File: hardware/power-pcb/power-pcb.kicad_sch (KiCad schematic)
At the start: 28 parts, among them J1 MicroFit3.0_1x2, J2 XT60PW-M-AS, J3 XT30, J4 XT30, K1 CB1-P-12V, Q1 SI4946CDY-T1-GE3, Q2 IRF4905, U1 LTC4365TS8, U2 TMCS1100A2QDR

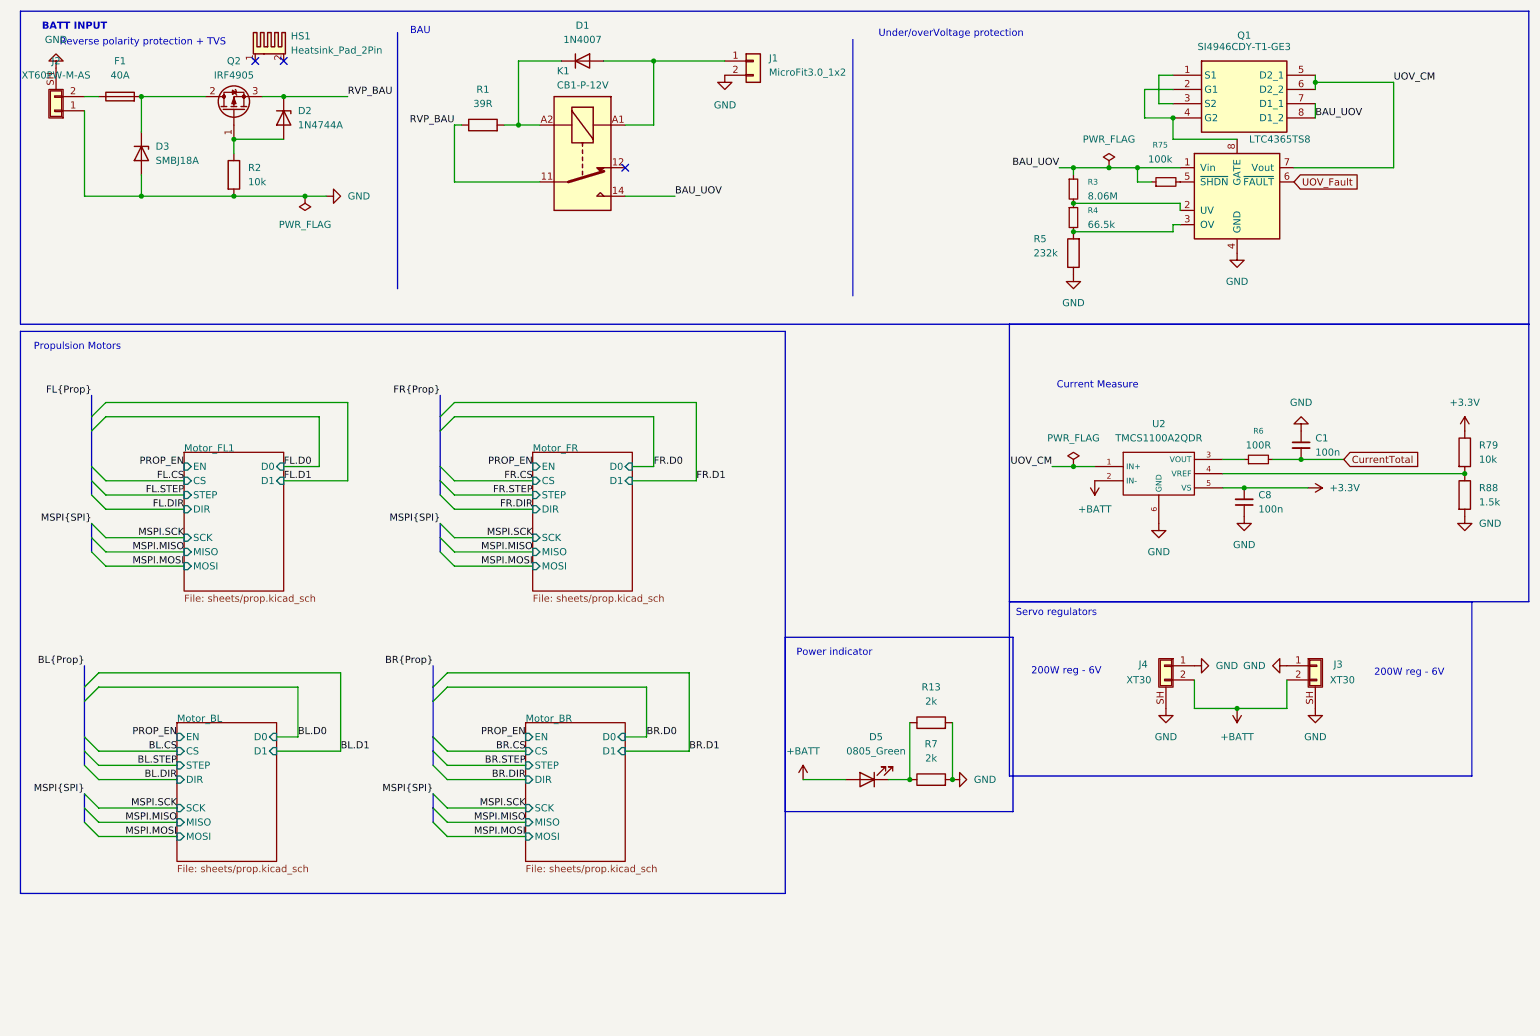
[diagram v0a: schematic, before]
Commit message: Added power pcb sch + design
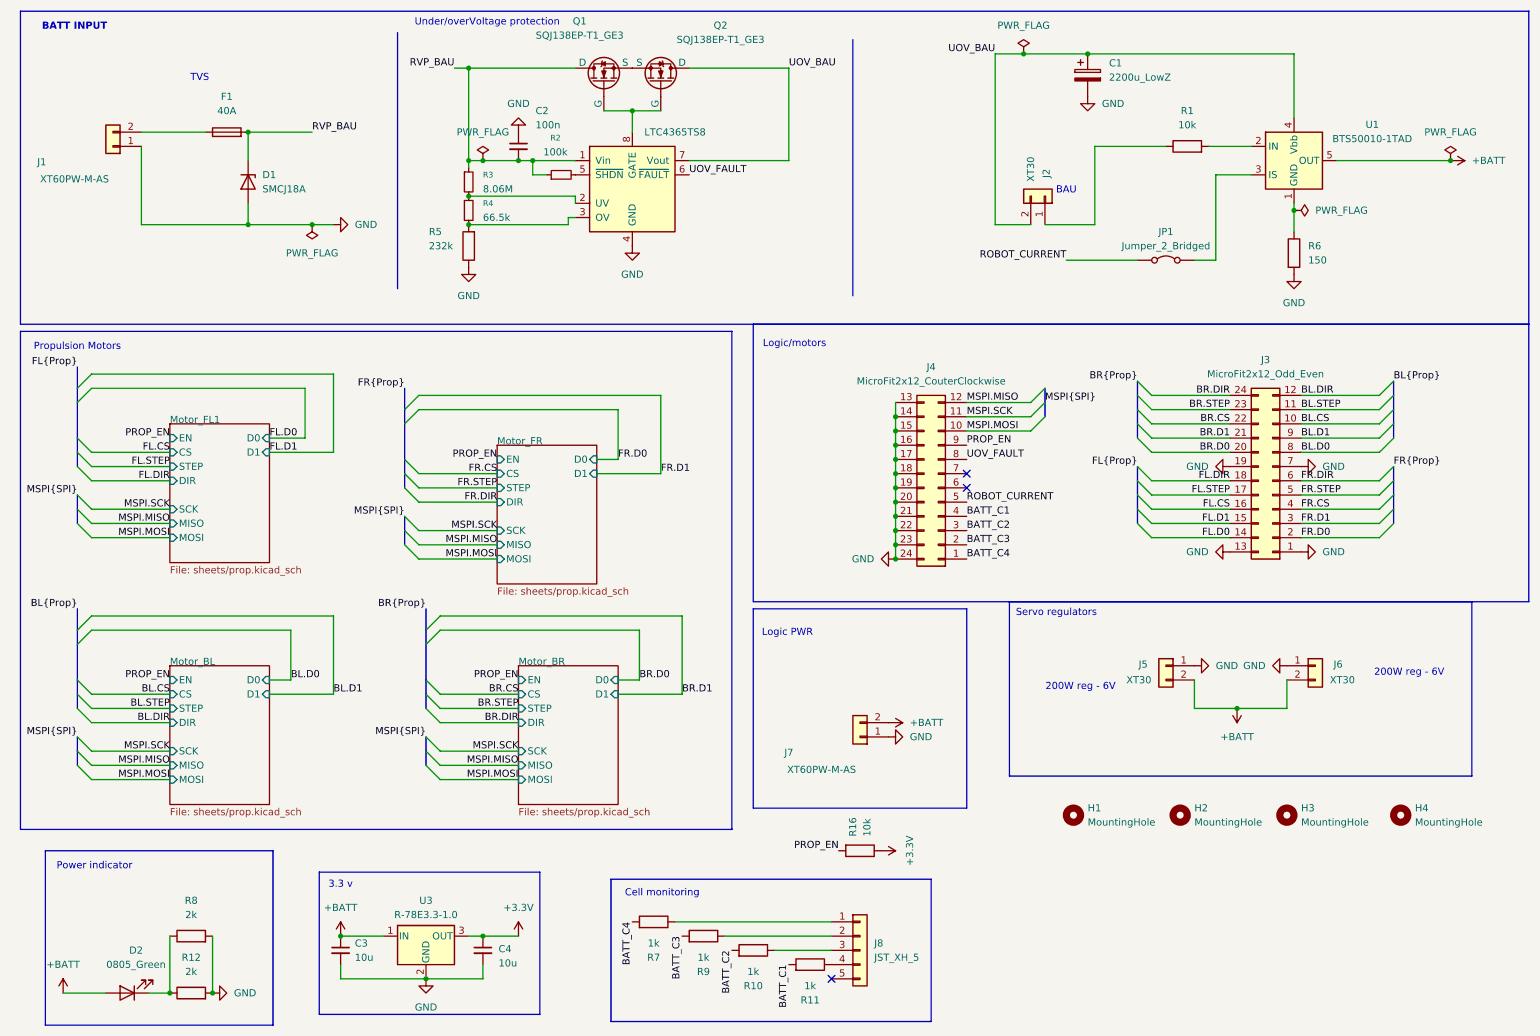
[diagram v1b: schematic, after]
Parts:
- removed C1, C8: 100n, Capacitor_SMD:C_0805_2012Metric_Pad1.18x1.45mm_HandSolder, symbol Device:C_Small
- removed D1: 1N4007, Diode_THT:D_DO-41_SOD81_P10.16mm_Horizontal, symbol Diode:1N4007
- removed D2: 1N4744A, Diode_THT:D_DO-41_SOD81_P10.16mm_Horizontal, symbol Diode:1N47xxA
- removed HS1: Heatsink_Pad_2Pin, Project:265118ABHE22, symbol Mechanical:Heatsink_Pad_2Pin
- removed J1: MicroFit3.0_1x2, Project:Molex_Micro-Fit_3.0_43650-0215_1x02_P3.00mm_Vertical, symbol Connector_Generic:Conn_01x02
- removed K1: CB1-P-12V, Project:CB1P12V, symbol Relay:Relay_SPDT
- removed Q1: SI4946CDY-T1-GE3, Package_SO:SO-8_3.9x4.9mm_P1.27mm, symbol Project:SISB46DN-T1-GE3
- removed Q2: IRF4905, Package_TO_SOT_THT:TO-220-3_Vertical, symbol Transistor_FET:IRF4905
- removed R2, R79: 10k, Resistor_SMD:R_0805_2012Metric_Pad1.20x1.40mm_HandSolder, symbol Device:R
- removed R6: 100R, Resistor_SMD:R_0805_2012Metric_Pad1.20x1.40mm_HandSolder, symbol Device:R_Small
- removed R88: 1.5k, Resistor_SMD:R_0805_2012Metric_Pad1.20x1.40mm_HandSolder, symbol Device:R
- removed U2: TMCS1100A2QDR, Project:TMCS1100A2QDR, symbol Project:TMCS1100A2QDR
- added C1: 2200u_LowZ, Capacitor_THT:CP_Radial_D16.0mm_P7.50mm, symbol Device:C_Polarized
- added C2: 100n, Capacitor_SMD:C_0805_2012Metric_Pad1.18x1.45mm_HandSolder, symbol Device:C_Small
- added C3, C4: 10u, Capacitor_SMD:C_0805_2012Metric_Pad1.18x1.45mm_HandSolder, symbol Device:C_Small
- added H1, H2, H3, H4: MountingHole, MountingHole:MountingHole_3.2mm_M3, symbol Mechanical:MountingHole
- added J2: XT30, Project:AMASS_XT30UPB-M_1x02_P5.0mm_Vertical, symbol Connector_Generic:Conn_01x02
- added J3: MicroFit2x12_Odd_Even, Project:Molex_Micro-Fit_3.0_43045-2412_2x12_P3.00mm_Vertical, symbol Connector_Generic:Conn_02x12_Top_Bottom
- added J4: MicroFit2x12_CouterClockwise, Project:Molex_Micro-Fit_3.0_43045-2412_2x12_P3.00mm_Vertical, symbol Connector_Generic:Conn_02x12_Counter_Clockwise
- added J7: XT60PW-M-AS, Connector_AMASS:AMASS_XT60-M_1x02_P7.20mm_Vertical, symbol Connector_Generic:Conn_01x02
- added J8: JST_XH_5, Project:JST_XH_B5B-XH-AM_1x05_P2.50mm_Vertical, symbol Connector_Generic:Conn_01x05
- added JP1: Jumper_2_Bridged, Project:TestPoint_2Pads_Pitch2.54mm_Drill0.8mm, symbol Jumper:Jumper_2_Bridged
- added Q1, Q2: SQJ138EP-T1_GE3, Project:PowerPAK_SO-8L_Single_MOS, symbol Simulation_SPICE:NMOS
- added R10, R11, R7, R9: 1k, Resistor_SMD:R_0805_2012Metric_Pad1.20x1.40mm_HandSolder, symbol Device:R
- added R16: 10k, Resistor_SMD:R_0805_2012Metric_Pad1.20x1.40mm_HandSolder, symbol Device:R
- added R6: 150, Resistor_SMD:R_0805_2012Metric_Pad1.20x1.40mm_HandSolder, symbol Device:R
- added U1: BTS50010-1TAD, Package_TO_SOT_SMD:TO-263-7_TabPin4, symbol Power_Management:BTS50010-1TAD
- added U3: R-78E3.3-1.0, Converter_DCDC:Converter_DCDC_RECOM_R-78E-0.5_THT, symbol Converter_DCDC:R-78E3.3-1.0
- D1: renamed from D3; value SMBJ18A -> SMCJ18A; footprint Diode_SMD:D_SMB_Handsoldering -> Diode_SMD:D_SMB-SMC_Universal_Handsoldering
- J1: renamed from J2; footprint Project:AMASS_XT60IPW-M_1x03_P7.20mm_Horizontal -> Connector_AMASS:AMASS_XT60-M_1x02_P7.20mm_Vertical; symbol Connector_Generic_Shielded:Conn_01x02_Shielded -> Connector_Generic:Conn_01x02
- J5: renamed from J4; footprint (none) -> Project:AMASS_XT30UPB-M_1x02_P5.0mm_Vertical; symbol Connector_Generic_Shielded:Conn_01x02_Shielded -> Connector_Generic:Conn_01x02
- J6: renamed from J3; footprint (none) -> Project:AMASS_XT30UPB-M_1x02_P5.0mm_Vertical; symbol Connector_Generic_Shielded:Conn_01x02_Shielded -> Connector_Generic:Conn_01x02
- R1: value 39R -> 10k; footprint Resistor_SMD:R_2512_6332Metric_Pad1.40x3.35mm_HandSolder -> Resistor_SMD:R_0805_2012Metric_Pad1.20x1.40mm_HandSolder
- renumbered D5 to D2, R7 to R12, R75 to R2, R13 to R8, U1 to U2
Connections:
- net BAU_UOV is gone; now on net RVP_BAU: R2.1, R3.1, U2.1 (Vin)
- net +3.3V: now also C4.1, R16.1, U3.3 (OUT)
- net +BATT: now also C3.1, J7.2 (Pin_2), U1.5 (OUT), U1.6 (OUT), U1.7 (OUT), U3.1 (IN)
- net BL.CS: now also J3.10 (Pin_10)
- net BL.D0: now also J3.8 (Pin_8)
- net BL.D1: now also J3.9 (Pin_9)
- net BL.DIR: now also J3.12 (Pin_12)
- net BL.STEP: now also J3.11 (Pin_11)
- net BR.CS: now also J3.22 (Pin_22)
- net BR.D0: now also J3.20 (Pin_20)
- net BR.D1: now also J3.21 (Pin_21)
- net BR.DIR: now also J3.24 (Pin_24)
- net BR.STEP: now also J3.23 (Pin_23)
- net FL.CS: now also J3.16 (Pin_16)
- net FL.D0: now also J3.14 (Pin_14)
- net FL.D1: now also J3.15 (Pin_15)
- net FL.DIR: now also J3.18 (Pin_18)
- net FL.STEP: now also J3.17 (Pin_17)
- net FR.CS: now also J3.4 (Pin_4)
- net FR.D0: now also J3.2 (Pin_2)
- net FR.D1: now also J3.3 (Pin_3)
- net FR.DIR: now also J3.6 (Pin_6)
- net FR.STEP: now also J3.5 (Pin_5)
- net GND: now also C1.2, C2.1, C3.2, C4.2, J3.1 (Pin_1), J3.13 (Pin_13), J3.19 (Pin_19), J3.7 (Pin_7), J4.13 (Pin_13), J4.14 (Pin_14), J4.15 (Pin_15), J4.16 (Pin_16), J4.17 (Pin_17), J4.18 (Pin_18), J4.19 (Pin_19), J4.20 (Pin_20), J4.21 (Pin_21), J4.22 (Pin_22), J4.23 (Pin_23), J4.24 (Pin_24), J7.1 (Pin_1), R6.2, U3.2 (GND); no longer J1.SH (Shield), J5.SH (Shield), J6.SH (Shield)
- net MSPI.MISO: now also J4.12 (Pin_12)
- net MSPI.MOSI: now also J4.10 (Pin_10)
- net MSPI.SCK: now also J4.11 (Pin_11)
- net PROP_EN: now also J4.9 (Pin_9), R16.2
- net RVP_BAU: now also D1.1 (K), F1.2, C2.2, Q1.1 (D); no longer R1.1
- net at R1.2: now also U1.2 (IN)
- net at U2.8 (GATE): now also Q1.2 (G), Q2.2 (G)
- net UOV_CM renamed UOV_BAU
- net UOV_BAU: now also C1.1, J2.2 (Pin_2), Q2.1 (D), U1.4 (Vbb)
- net UOV_Fault renamed UOV_FAULT
- net UOV_FAULT: now also J4.8 (Pin_8)
- new net: J8.4 (Pin_4), R11.1
- new net: R6.1, U1.1 (GND)
- new net: Q1.3 (S), Q2.3 (S)
- new net: J8.1 (Pin_1), R7.1
- new net: J8.2 (Pin_2), R9.1
- new net: J8.3 (Pin_3), R10.1
- new net: JP1.2 (B), U1.3 (IS)
- new net: J2.1 (Pin_1), R1.1
- new net BATT_C1: J4.4 (Pin_4), R11.2
- new net BATT_C2: J4.3 (Pin_3), R10.2
- new net BATT_C3: J4.2 (Pin_2), R9.2
- new net BATT_C4: J4.1 (Pin_1), R7.2
- new net ROBOT_CURRENT: J4.5 (Pin_5), JP1.1 (A)
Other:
- note added: "3.3 v"
- note added: "Cell monitoring"
- note added: "Logic PWR"
- note added: "Logic/motors"
- note added: "TVS"
- note removed: "Current Measure"
- note removed: "Reverse polarity protection + TVS"
- moved on the sheet: D1, D2, F1, R12, R2, R3, R4, R5, R8
